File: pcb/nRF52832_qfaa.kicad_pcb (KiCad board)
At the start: 4 copper layers, 41.5 x 13 mm, 87 parts, among them J1 Conn_01x01_Female, J2 Conn_02x05_Odd_Even, U1 NRF52832, U2 W25Q32JVZP, U3 TPS63802DLAR, U4 BQ24078RGTR, U5 RV-4162-C7, U6 SN74LVC1G79DBVT, X1 32.768kHz, X2 32MHz

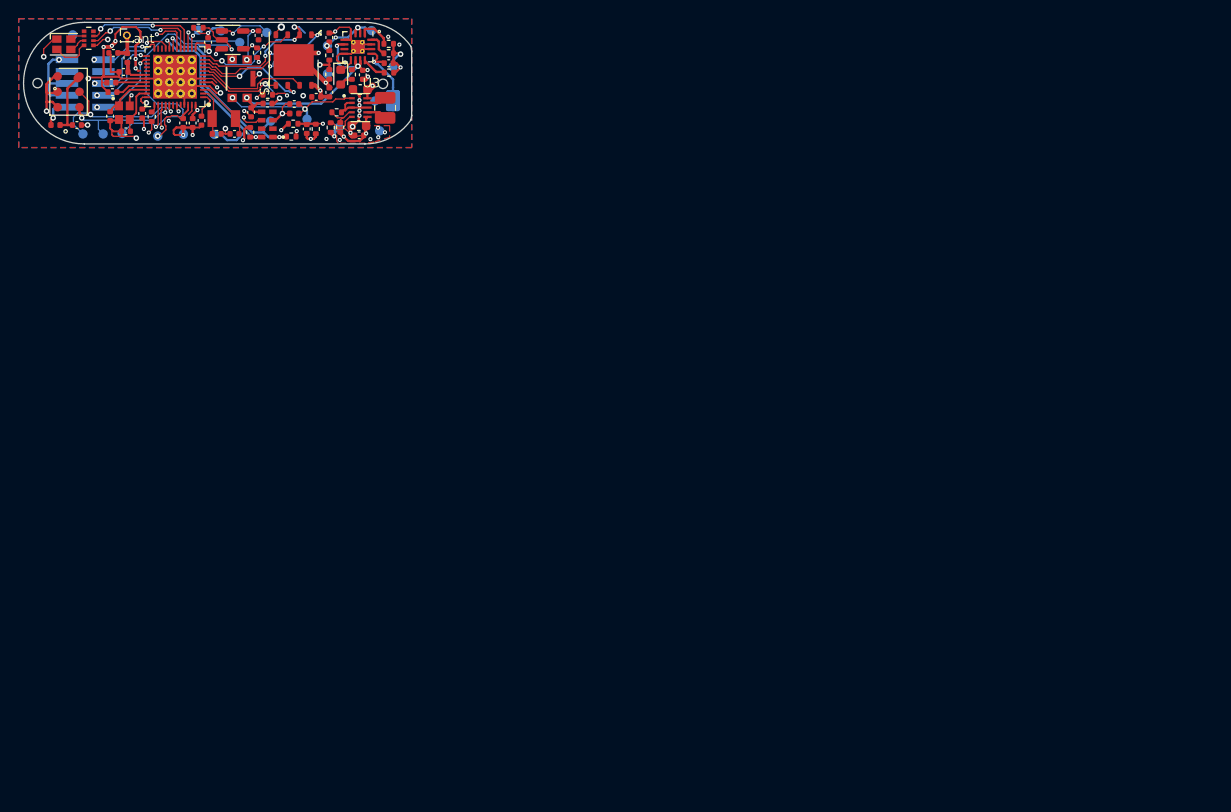
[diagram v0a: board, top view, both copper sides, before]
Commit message: start laying out 1.4
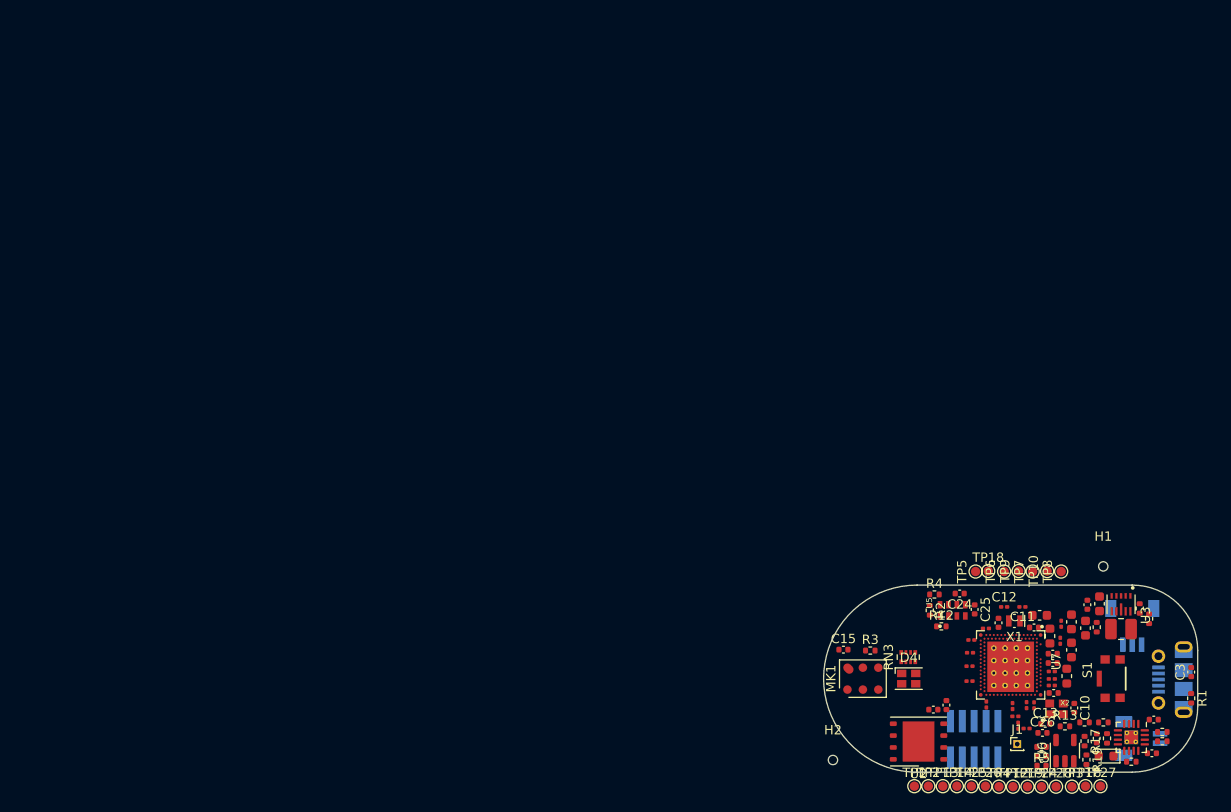
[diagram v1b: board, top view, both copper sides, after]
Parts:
- removed C14: 0.8pF, Capacitor_SMD:C_0402_1005Metric
- removed C16, C6, C9: 100nF, Capacitor_SMD:C_0402_1005Metric
- removed C22: DNP, Capacitor_SMD:C_0402_1005Metric
- removed C4: 1µF, Capacitor_SMD:C_0402_1005Metric
- removed C5: 4.7µF, Capacitor_SMD:C_0402_1005Metric
- removed C7: 100pF, Capacitor_SMD:C_0402_1005Metric
- removed C8: N.M., Capacitor_SMD:C_0402_1005Metric
- removed D1: ASMB-LTC2-0A335, nRF52832_qfaa:LED_Cree-PLCC4_2x2mm_CW
- removed L2: 3.3nH, Capacitor_SMD:C_0402_1005Metric
- removed RN1: R_Pack04, Resistor_SMD:R_Array_Convex_4x0402
- removed TP11: TestPoint, TestPoint:TestPoint_Pad_D1.0mm
- removed U1: NRF52832, nRF52832_qfaa:QFN40P600X600X90-48_N
- added C28: 100n, Capacitor_SMD:C_0201_0603Metric, F.Cu at (130.8, 94.9)
- added C29: 100n, Capacitor_SMD:C_0201_0603Metric, F.Cu at (139.4, 98.2)
- added C30: 100n, Capacitor_SMD:C_0201_0603Metric, F.Cu at (132.4, 101.8)
- added C31: 100n, Capacitor_SMD:C_0201_0603Metric, F.Cu at (135.2, 101.9)
- added C32: 100n, Capacitor_SMD:C_0201_0603Metric, F.Cu at (132.4, 93.6)
- added C33: 100n, Capacitor_SMD:C_0201_0603Metric, F.Cu at (130.6, 99.3)
- added C34: 100n, Capacitor_SMD:C_0201_0603Metric, F.Cu at (130.6, 97.7)
- added C35: 100n, Capacitor_SMD:C_0201_0603Metric, F.Cu at (130.7, 96.2)
- added C36: N.C, Capacitor_SMD:C_0201_0603Metric, F.Cu at (137.5, 101.9)
- added C37: 1u, Capacitor_SMD:C_0402_1005Metric, F.Cu at (137.5, 93.5)
- added C38: 1u, Capacitor_SMD:C_0402_1005Metric, F.Cu at (139.6, 100.5)
- added C39: 1u, Capacitor_SMD:C_0402_1005Metric, F.Cu at (133.7, 93.0)
- added C39(NP0)1: 100pF, Capacitor_SMD:C_0201_0603Metric, F.Cu at (139.4, 99.7)
- added C40: 1u, Capacitor_SMD:C_0402_1005Metric, F.Cu at (139.5, 97.3)
- added C41: 2.2u, Capacitor_SMD:C_0603_1608Metric, F.Cu at (138.1, 92.2)
- added C42: 4.7u, Capacitor_SMD:C_0603_1608Metric, F.Cu at (141.5, 95.9)
- added C43: 4.7u, Capacitor_SMD:C_0603_1608Metric, F.Cu at (141.5, 92.9)
- added C44: 1u, Capacitor_SMD:C_0402_1005Metric, F.Cu at (139.5, 96.3)
- added C45: 100n, Capacitor_SMD:C_0201_0603Metric, F.Cu at (139.4, 99.0)
- added C46: DNP, Capacitor_SMD:C_0201_0603Metric, F.Cu at (136.7, 104.3)
- added C47: 0.7pF, Capacitor_SMD:C_0201_0603Metric, F.Cu at (135.5, 103.0)
- added D4: ASMB-LTC2-0A335, nRF52832_qfaa:LED_Cree-PLCC4_2x2mm_CW, F.Cu at (124.1, 99.0)
- added J3: USB_B_Micro, Connector_USB:USB_Micro-B_Molex-105017-0001, B.Cu at (152.3, 99.1)
- added J4: Conn_01x02_Socket, _other:SM02B-SRSS-TB_LF__SN_, B.Cu at (149.0, 105.4)
- added J5: Conn_01x03_Socket, _other:JST_SM03B-SRSS-TB_LF__SN_, B.Cu at (148.0, 95.4)
- added L3: 10uH, Inductor_SMD:L_0603_1608Metric, F.Cu at (141.0, 98.7)
- added L4: 10uH, Inductor_SMD:L_0603_1608Metric, F.Cu at (139.2, 94.4)
- added L5: 15nH, Inductor_SMD:L_0201_0603Metric, F.Cu at (136.7, 101.8)
- added L6: 15nH, Inductor_SMD:L_0201_0603Metric, F.Cu at (140.3, 95.0)
- added L7: 2.2nH, Inductor_SMD:L_0201_0603Metric, F.Cu at (135.8, 104.0)
- added R20: 4.7, Resistor_SMD:R_0201_0603Metric, F.Cu at (140.4, 93.1)
- added RN3: R_Pack04, Resistor_SMD:R_Array_Convex_4x0402, F.Cu at (124.0, 96.7)
- added U7: NRF5340-QKAA-R7, _other:XCVR_NRF5340-QKAA-R7, F.Cu at (135.0, 97.5)
- C11, C12: footprint Capacitor_SMD:C_0402_1005Metric -> Capacitor_SMD:C_0201_0603Metric
- TP1, TP10, TP12, TP13, TP14, TP16, TP18, TP19, TP2, TP24, TP25, TP26, TP27, TP28, TP3, TP4, TP5, TP6, TP7, TP8, TP9: moved to F.Cu
- X1: footprint nRF52832_qfaa:XTAL_3215_N -> Crystal:Crystal_SMD_MicroCrystal_CM9V-T1A-2Pin_1.6x1.0mm
- moved TP19 129.9 mm to (136.8, 110.5), turned to 0 degrees
- moved R19 123.0 mm to (143.1, 107.7), turned to -90 degrees
- moved J1 121.7 mm to (135.7, 106.0)
- moved C13 119.2 mm to (138.7, 103.8), turned to 0 degrees
- moved C10 118.7 mm to (141.8, 102.1), turned to -90 degrees
- moved X2 118.3 mm to (139.9, 102.2), turned to 0 degrees
- moved J2 118.1 mm to (131.1, 105.5), turned to -90 degrees
- moved R13 117.4 mm to (140.8, 104.1), turned to 0 degrees
- moved U6 117.0 mm to (140.8, 106.7), turned to 90 degrees
- moved TP28 116.5 mm to (139.8, 110.5), turned to 0 degrees
- moved R17 115.1 mm to (142.9, 105.7), turned to -90 degrees
- moved R1 114.5 mm to (154.3, 101.1), turned to -90 degrees
- moved C20 114.4 mm to (150.3, 103.4), turned to 180 degrees
- moved C3 113.5 mm to (154.3, 98.3), turned to 90 degrees
- moved TP12 113.4 mm to (135.2, 110.5), turned to 0 degrees
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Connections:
- net /P0.00/XL1 renamed Net-(U7C-P0.00/XL1)
- net /P0.01/XL2 renamed Net-(U7C-P0.01/XL2)
- net /P0.28 renamed /PDM_CLK
- net /P0.29 renamed /PDM_DATA
- J2 pad 6: /P0.18/SWO -> /SWO
- R13 pad 1: /P0.25 -> unconnected-(R13-Pad1)
- TP6 pad 1: /P0.12 -> /UART_RX
- TP7 pad 1: /P0.11 -> /UART_TX
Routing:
- net GND: track 132.7 -> 0.00 mm, vias 41 -> 0
- net VCC: track 89.2 -> 0.00 mm, vias 17 -> 0
- net VSS: track 51.1 -> 0.00 mm, vias 8 -> 0
- net FF_CLK: track 34.4 -> 0.00 mm, vias 2 -> 0
- net MAIN_BUTTON: track 33.1 -> 0.00 mm, vias 5 -> 0
- net /Power/FF_D: track 24.8 -> 0.00 mm, vias 2 -> 0
- net /I2C_SCL: track 21.9 -> 0.00 mm, vias 2 -> 0
- net /I2C_SDA: track 21.8 -> 0.00 mm, vias 2 -> 0
- net /SWDCLK: track 19.1 -> 0.00 mm, vias 2 -> 0
- net /SWDIO: track 19.0 -> 0.00 mm, vias 2 -> 0
- net /PDM_DATA: track 17.3 -> 0.00 mm, vias 2 -> 0
- net MCU_POWER_LATCH: track 17.2 -> 0.00 mm, vias 2 -> 0
- net V_charger: track 16.5 -> 0.00 mm, vias 1 -> 0
- net VBAT_LEVEL: track 16.0 -> 0.00 mm, vias 2 -> 0
- net /MEM_CS: track 15.6 -> 0.00 mm, vias 2 -> 0
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- removed copper zone on B.Cu, net GND
- removed copper zone on F.Cu, net GND
- removed copper zone on In1.Cu, net GND
- removed copper zone on F.Cu, net VCC
- removed copper zone on In2.Cu, net VCC
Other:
- board size 41.5 x 13 mm -> 40 x 20 mm
- board text removed: "ant"
